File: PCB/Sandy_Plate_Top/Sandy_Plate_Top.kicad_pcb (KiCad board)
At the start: 2 copper layers, 285 x 37 mm, 21 parts

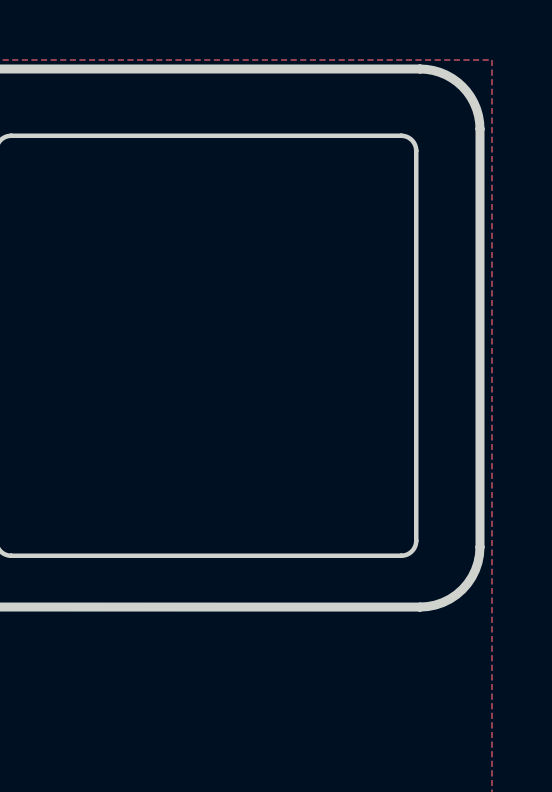
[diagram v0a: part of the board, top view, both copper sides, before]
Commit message: ERC, DRCチェック
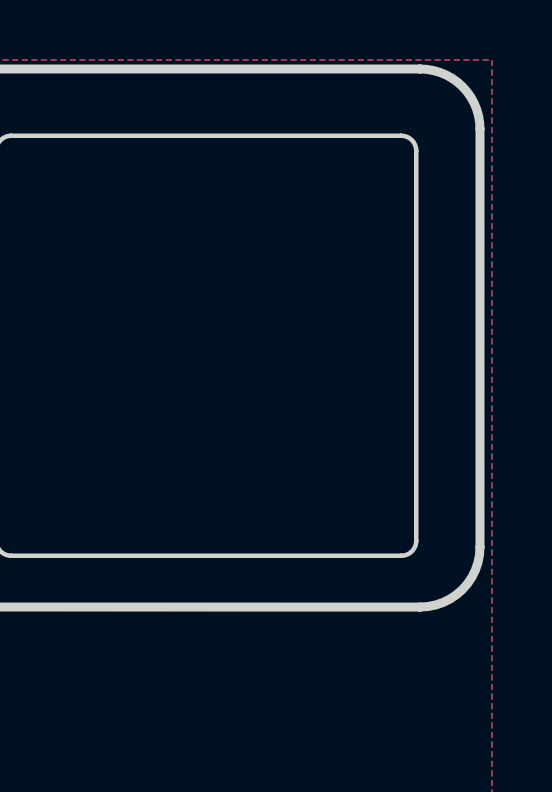
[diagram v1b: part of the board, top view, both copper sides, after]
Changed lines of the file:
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@@
     (fp_arc (start 140.35 -3.025) (mid 140.203553 -2.671447) (end 139.85 -2.525)
       (stroke (width 0.15) (type solid)) (layer "Edge.Cuts"))
-    (fp_arc (start 140.475 -18.75004) (mid 141.889257 -18.164285) (end 142.475 -16.75004)
+    (fp_arc (start 140.475 -18.75004) (mid 141.889222 -18.164279) (end 142.475 -16.75004)
       (stroke (width 0.3) (type solid)) (layer "Edge.Cuts"))
-    (fp_arc (start 142.475 -2.814254) (mid 141.889203 -1.400035) (end 140.475 -0.814254)
+    (fp_arc (start 142.475 -2.814254) (mid 141.889197 -1.40007) (end 140.475 -0.814254)
       (stroke (width 0.3) (type solid)) (layer "Edge.Cuts"))
     (group "" (id b45a4e6d-43e9-43f3-99a8-109a97b956a9)
